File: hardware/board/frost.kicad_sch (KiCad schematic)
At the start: 1 part, among them U1 RK3568

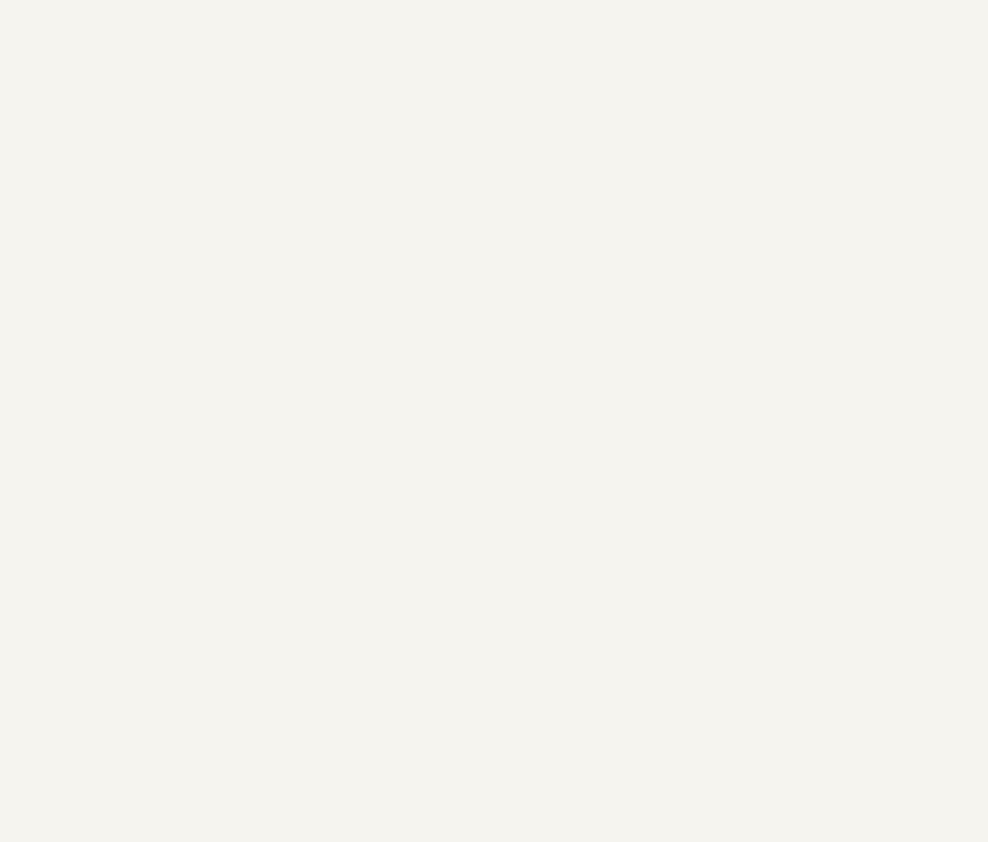
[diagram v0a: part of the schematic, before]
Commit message: sensors
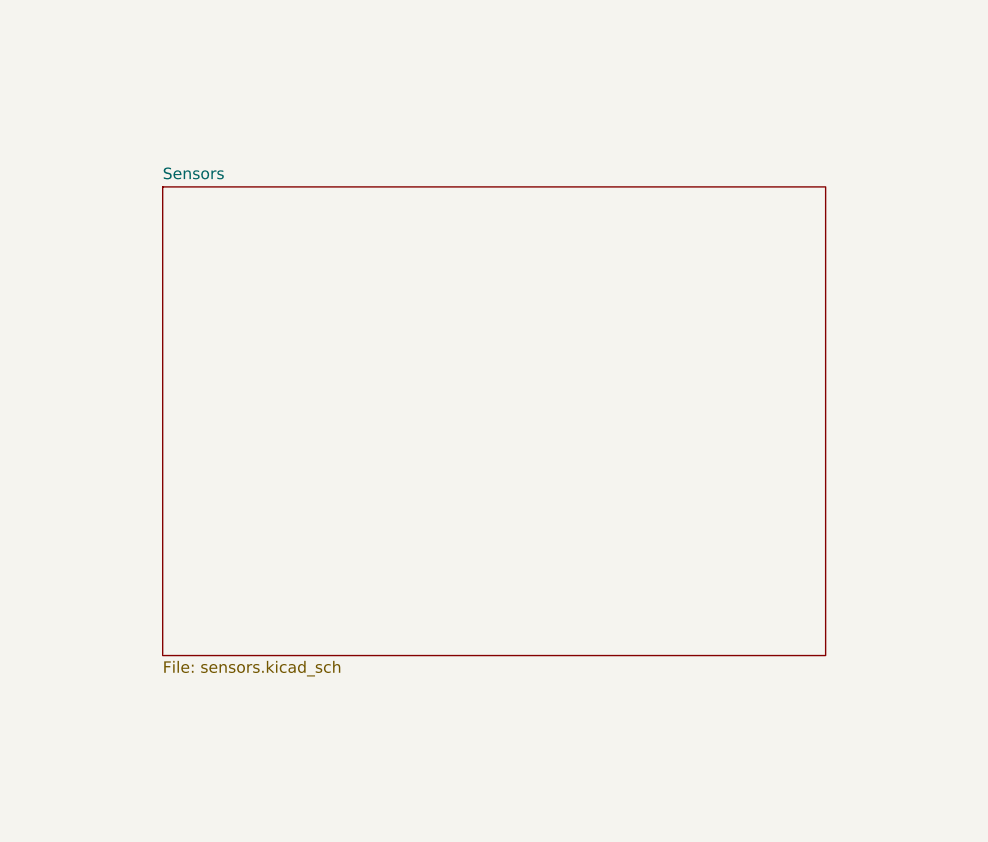
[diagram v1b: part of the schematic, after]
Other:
- added sheet Sensors (sensors.kicad_sch)
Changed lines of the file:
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@@
+	)
+	(sheet
+		(at 396.24 398.78)
+		(size 73.66 52.07)
+		(exclude_from_sim no)
+		(in_bom yes)
+		(on_board yes)
+		(dnp no)
+		(fields_autoplaced yes)
+		(stroke
+			(width 0.1524)
+			(type solid)
+		)
+		(fill
+			(color 0 0 0 0.0000)
+		)
+		(property "Sheetname" "Sensors"
+			(at 396.24 398.0684 0)
+			(effects
+				(font
+					(size 1.27 1.27)
+				)
+				(justify left bottom)
+			)
+		)
+		(property "Sheetfile" "sensors.kicad_sch"
+			(at 396.24 451.4346 0)
+			(effects
+				(font
+					(size 1.27 1.27)
+				)
+				(justify left top)
+			)
+		)
+		(instances
+			(project "frost"
+				(path "/3bc38516-4fe0-4022-adb8-9fd55b66cd2d"
+					(page "12")
+				)
+			)
+		)
 	)
 	(sheet

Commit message: finished schematic!
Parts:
- removed unit 15 of U1
- removed unit 10 of U1
- removed unit 17 of U1
- removed unit 22 of U1
- removed unit 11 of U1
- removed unit 12 of U1
- removed unit 14 of U1
- removed unit 21 of U1
- removed unit 7 of U1
- removed unit 8 of U1
- removed unit 9 of U1
- removed unit 20 of U1
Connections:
- no-connect marks 0 -> 24
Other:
- moved on the sheet: U1R, U1S
